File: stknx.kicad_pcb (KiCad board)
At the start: 2 copper layers, 51.3 x 20.3 mm, 51 parts, among them J1 KNX, J2 PMOD, J3 VDDHV, J4 VCCCORE, J5 VDCDC, U1 STKNX

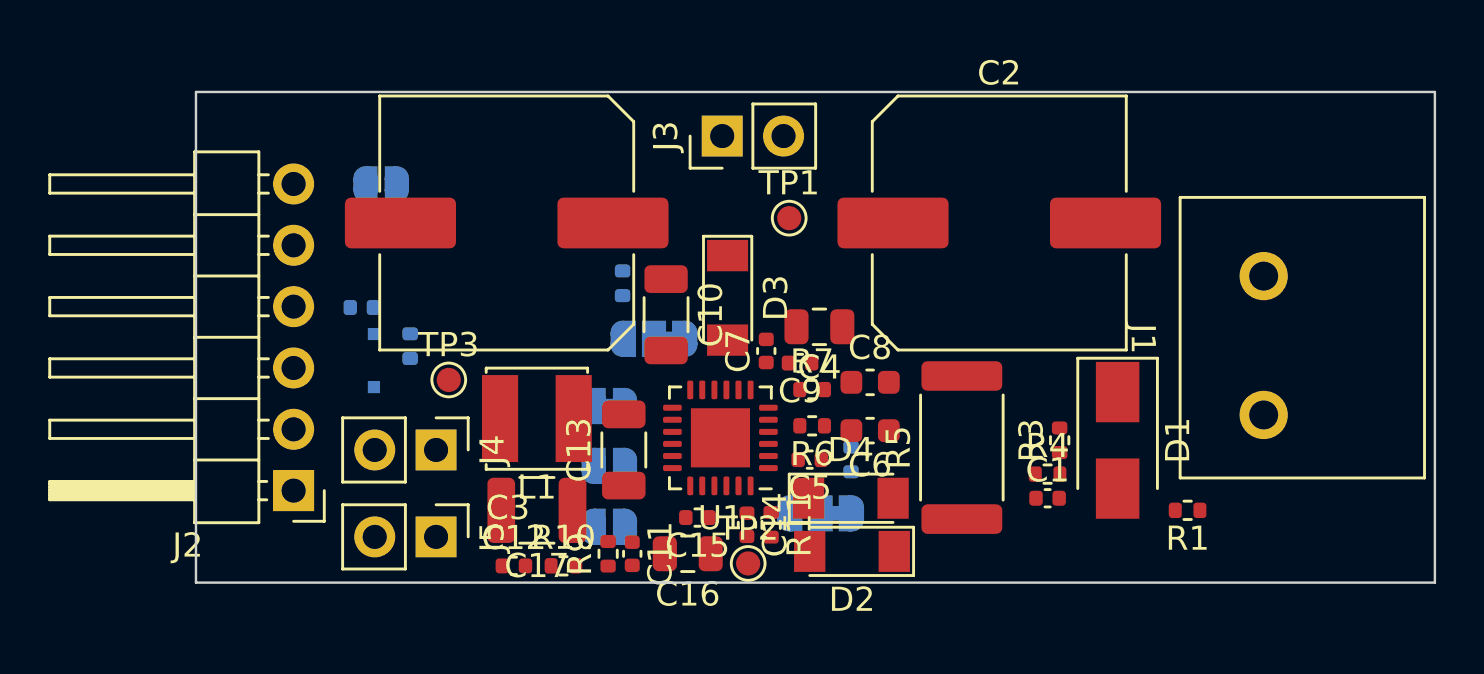
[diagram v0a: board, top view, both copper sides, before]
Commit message: First attempts at routing
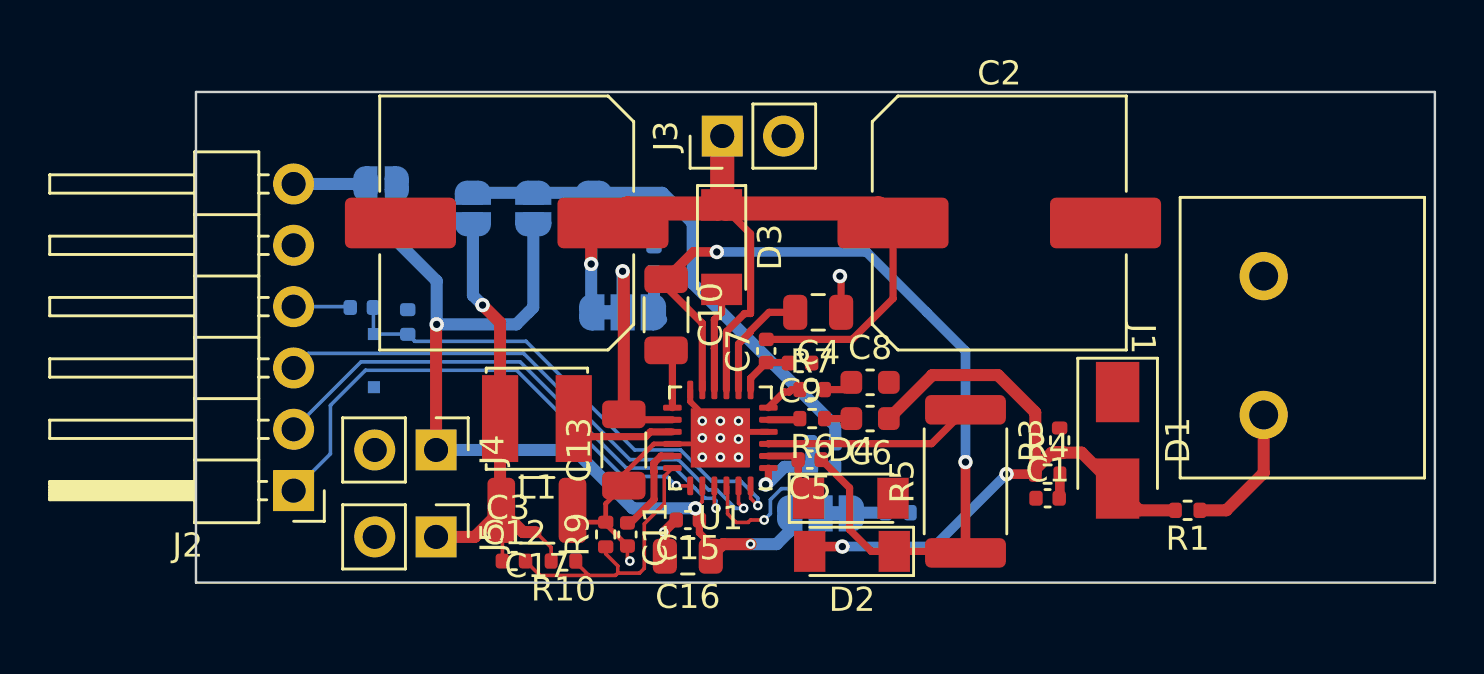
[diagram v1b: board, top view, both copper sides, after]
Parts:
- removed TP1: HV, TestPoint:TestPoint_Pad_D1.0mm
- removed TP2: VCCCORE, TestPoint:TestPoint_Pad_D1.0mm
- removed TP3: VCCDCDC, TestPoint:TestPoint_Pad_D1.0mm
- C14, R11: moved to B.Cu
- moved JP3 14.3 mm to (165.9, 101.6), turned to -90 degrees
- moved JP4 11.1 mm to (168.4, 101.6), turned to -90 degrees
- moved JP2 8.21 mm to (170.9, 101.6), turned to -90 degrees
- moved R11 4.02 mm to (180.4, 111.3), turned to 0 degrees
- moved C14 3.96 mm to (180.4, 112.3), turned to 0 degrees
- moved R8 2.94 mm to (183.5, 114.2), turned to 180 degrees
- moved D3 2.11 mm to (176.2, 103.2)
- moved JP1 1.70 mm to (172.1, 105.9), turned to 0 degrees
- moved R2 1.64 mm to (173.4, 103.7)
- moved R5 1.41 mm to (186.3, 112.9)
- moved R12 1.00 mm to (163.2, 106.3), turned to 90 degrees
- moved C11 0.82 mm to (172.3, 115.1)
- moved R9 0.81 mm to (171.4, 115.1)
- moved C4 0.60 mm to (180.2, 105.9)
- moved C6 0.50 mm to (182.3, 110.3)
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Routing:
- net /VCCCORE: track 0.00 -> 38.9 mm, vias 0 -> 3
- net /VDDHV: track 0.00 -> 38.6 mm, vias 0 -> 1
- net Net-(C10-Pad1): track 0.00 -> 36.7 mm, vias 0 -> 2
- net Net-(C6-Pad1): track 0.00 -> 27.9 mm, vias 0 -> 2
- net /KNX_RX: track 0.00 -> 22.6 mm, vias 0 -> 1
- net /KNX_OK: track 0.00 -> 22.3 mm, vias 0 -> 1
- net /KNX_VCC_OK: track 0.00 -> 21.6 mm, vias 0 -> 1
- net /VDD_REGIN: track 0.00 -> 21.2 mm
- net Net-(C18-Pad1): track 0.00 -> 21.1 mm, vias 0 -> 1
- net /VDCDC: track 0.00 -> 20.9 mm, vias 0 -> 1
- net GND: track 0.00 -> 17.4 mm, vias 0 -> 12
- net Net-(C12-Pad2): track 0.00 -> 12.2 mm
- net /DCDC_IN: track 0.00 -> 9.75 mm, vias 0 -> 1
- net Net-(R5-Pad2): track 0.00 -> 8.75 mm
- net /VCC_SEL: track 0.00 -> 7.05 mm, vias 0 -> 1
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- added copper zone on B.Cu, net GND
- added copper zone on F.Cu, net GND
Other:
- rule pad_to_mask_clearance: 0 -> 0.05

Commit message: Minor fixes
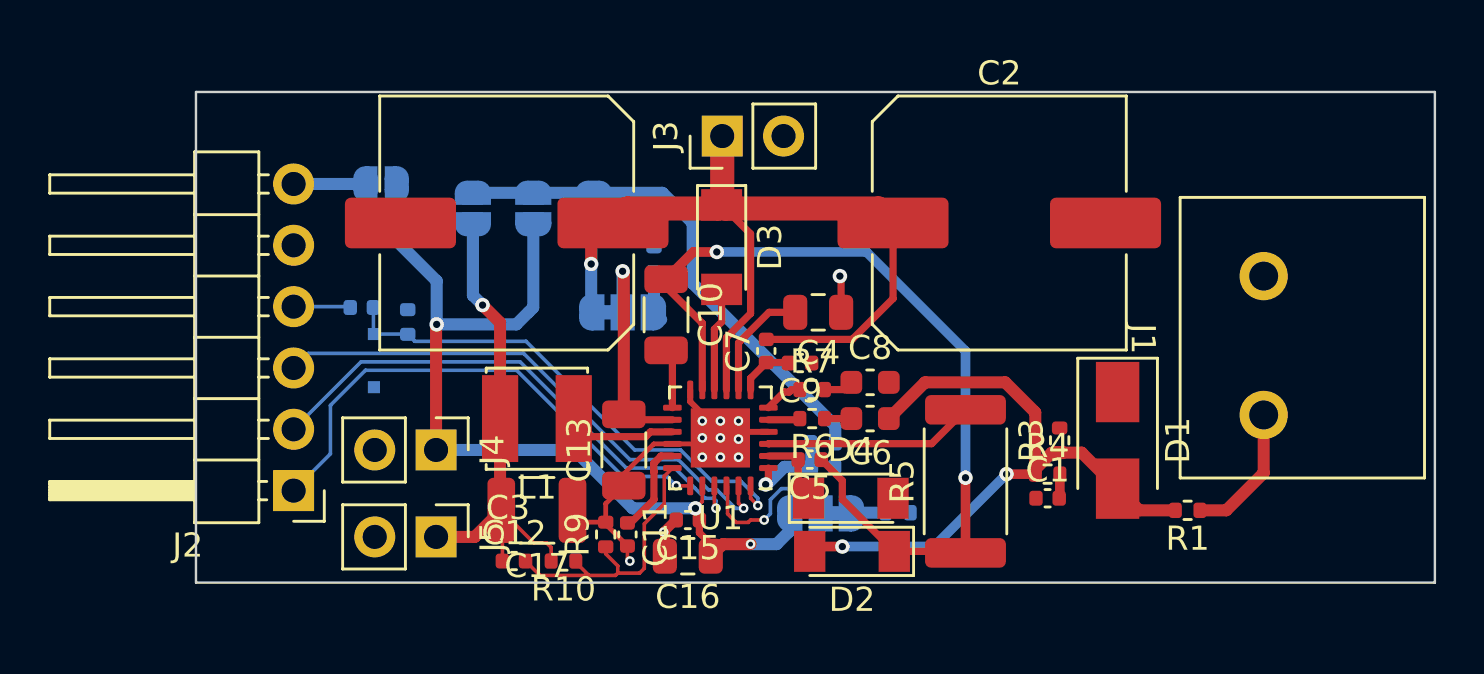
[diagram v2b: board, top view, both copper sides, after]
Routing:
- net Net-(C10-Pad1): track 36.7 -> 36.2 mm
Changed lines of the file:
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@@
   (segment (start 176.35 101.6) (end 176.2 101.45) (width 1) (layer "F.Cu") (net 3))
   (segment (start 183.3 102.2) (end 182.7 101.6) (width 1) (layer "F.Cu") (net 3))
+  (segment (start 176.4 109.1125) (end 176.4 106.95) (width 0.3) (layer "F.Cu") (net 3))
   (segment (start 183.3 105.329776) (end 183.3 102.2) (width 0.3) (layer "F.Cu") (net 3))
-  (segment (start 176.4 109.1125) (end 176.4 106.7) (width 0.3) (layer "F.Cu") (net 3))
+  (segment (start 177.399511 105.950489) (end 177.399511 102.649511) (width 0.3) (layer "F.Cu") (net 3))
   (segment (start 172.3 101.6) (end 176.05 101.6) (width 1) (layer "F.Cu") (net 3))
-  (segment (start 177.399511 105.949511) (end 177.399511 102.649511) (width 0.3) (layer "F.Cu") (net 3))
   (segment (start 170.8 103.9) (end 170.8 103.1) (width 0.5) (layer "F.Cu") (net 3))
+  (segment (start 177.399511 102.649511) (end 176.2 101.45) (width 0.3) (layer "F.Cu") (net 3))
   (segment (start 182.7 101.6) (end 176.35 101.6) (width 1) (layer "F.Cu") (net 3))
-  (segment (start 177.399511 102.649511) (end 176.2 101.45) (width 0.3) (layer "F.Cu") (net 3))
   (segment (start 170.8 103.1) (end 171.7 102.2) (width 0.5) (layer "F.Cu") (net 3))
-  (segment (start 177.150489 105.949511) (end 177.399511 105.949511) (width 0.3) (layer "F.Cu") (net 3))
-  (segment (start 176.4 106.7) (end 177.150489 105.949511) (width 0.3) (layer "F.Cu") (net 3))
   (segment (start 178.05 107.02) (end 181.609776 107.02) (width 0.3) (layer "F.Cu") (net 3))
+  (segment (start 176.4 106.95) (end 177.399511 105.950489) (width 0.3) (layer "F.Cu") (net 3))
   (segment (start 176.05 101.6) (end 176.2 101.45) (width 1) (layer "F.Cu") (net 3))
   (segment (start 176.225 98.6) (end 176.225 101.425) (width 1) (layer "F.Cu") (net 3))
@@
   (segment (start 170.8 105.9) (end 170.8 102.35) (width 0.5) (layer "B.Cu") (net 3))
   (segment (start 170.8 102.35) (end 170.9 102.25) (width 0.5) (layer "B.Cu") (net 3))
-  (segment (start 177.39048 106.673354) (end 178.163834 105.9) (width 0.3) (layer "F.Cu") (net 4))
-  (segment (start 176.9 107.206416) (end 177.39048 106.715936) (width 0.3) (layer "F.Cu") (net 4))
-  (segment (start 176.9 109.1125) (end 176.9 107.206416) (width 0.3) (layer "F.Cu") (net 4))
+  (segment (start 179.05 106.1) (end 179.25 105.9) (width 0.3) (layer "F.Cu") (net 4))
   (segment (start 178.163834 105.9) (end 179.25 105.9) (width 0.3) (layer "F.Cu") (net 4))
-  (segment (start 177.39048 106.715936) (end 177.39048 106.673354) (width 0.3) (layer "F.Cu") (net 4))
-  (segment (start 179.05 106.1) (end 179.25 105.9) (width 0.3) (layer "F.Cu") (net 4))
+  (segment (start 176.9 109.1125) (end 176.9 107.163834) (width 0.3) (layer "F.Cu") (net 4))
+  (segment (start 176.9 107.163834) (end 178.163834 105.9) (width 0.3) (layer "F.Cu") (net 4))
   (segment (start 186.2375 115.8) (end 186.3 115.8625) (width 0.3) (layer "F.Cu") (net 5))
   (segment (start 175.025 103.4) (end 173.9 104.525) (width 0.4) (layer "F.Cu") (net 5))
-  (segment (start 181.5 114.9) (end 182.4 115.8) (width 0.3) (layer "F.Cu") (net 5))
   (segment (start 183.35 115.8) (end 186.2375 115.8) (width 0.3) (layer "F.Cu") (net 5))
   (segment (start 173.9 104.849022) (end 173.9 104.525) (width 0.3) (layer "F.Cu") (net 5))
-  (segment (start 182.4 115.8) (end 183.35 115.8) (width 0.3) (layer "F.Cu") (net 5))
-  (segment (start 186.3 115.8625) (end 186.3 112.1) (width 0.4) (layer "F.Cu") (net 5))
-  (segment (start 180.33 112) (end 181.5 113.17) (width 0.3) (layer "F.Cu") (net 5))
+  (segment (start 181.2 112.87) (end 181.2 113.65) (width 0.3) (layer "F.Cu") (net 5))
   (segment (start 175.4 109.1125) (end 175.4 106.349022) (width 0.3) (layer "F.Cu") (net 5))
+  (segment (start 186.3 115.8625) (end 186.3 112.75) (width 0.4) (layer "F.Cu") (net 5))
   (segment (start 175.4 106.349022) (end 173.9 104.849022) (width 0.3) (layer "F.Cu") (net 5))
   (segment (start 176 103.4) (end 175.025 103.4) (width 0.4) (layer "F.Cu") (net 5))
-  (segment (start 181.5 113.17) (end 181.5 114.9) (width 0.3) (layer "F.Cu") (net 5))
-  (via (at 186.3 112.1) (size 0.6) (drill 0.3) (layers "F.Cu" "B.Cu") (net 5))
+  (segment (start 181.2 113.65) (end 183.35 115.8) (width 0.3) (layer "F.Cu") (net 5))
+  (segment (start 180.33 112) (end 181.2 112.87) (width 0.3) (layer "F.Cu") (net 5))
+  (via (at 186.3 112.75) (size 0.6) (drill 0.3) (layers "F.Cu" "B.Cu") (net 5))
   (via (at 176 103.4) (size 0.6) (drill 0.3) (layers "F.Cu" "B.Cu") (net 5))
-  (segment (start 182.2 103.4) (end 176 103.4) (width 0.4) (layer "B.Cu") (net 5))
-  (segment (start 184.7 105.9) (end 182.2 103.4) (width 0.4) (layer "B.Cu") (net 5))
-  (segment (start 186.3 112.1) (end 186.3 107.5) (width 0.4) (layer "B.Cu") (net 5))
-  (segment (start 186.3 107.5) (end 184.7 105.9) (width 0.4) (layer "B.Cu") (net 5))
+  (segment (start 176 103.4) (end 182.2 103.4) (width 0.4) (layer "B.Cu") (net 5))
+  (segment (start 186.3 107.5) (end 186.3 112.75) (width 0.4) (layer "B.Cu") (net 5))
+  (segment (start 182.2 103.4) (end 186.3 107.5) (width 0.4) (layer "B.Cu") (net 5))
   (segment (start 179.37 112) (end 179.37 113.17) (width 0.3) (layer "F.Cu") (net 6))
   (segment (start 179.22 111.85) (end 179.37 112) (width 0.3) (layer "F.Cu") (net 6))
@@
   (segment (start 188 112.6) (end 189.19 112.6) (width 0.4) (layer "F.Cu") (net 7))
   (segment (start 189.880001 111.71) (end 189.19 112.400001) (width 0.5) (layer "F.Cu") (net 7))
-  (segment (start 184.925 108.5) (end 183.125 110.3) (width 0.5) (layer "F.Cu") (net 7))
+  (segment (start 184.625 108.8) (end 183.125 110.3) (width 0.5) (layer "F.Cu") (net 7))
   (segment (start 194.99 114.1) (end 193.5 114.1) (width 0.5) (layer "F.Cu") (net 7))
+  (segment (start 189.19 110.043802) (end 187.946198 108.8) (width 0.5) (layer "F.Cu") (net 7))
+  (segment (start 191.11 111.71) (end 190.2 111.71) (width 0.5) (layer "F.Cu") (net 7))
   (segment (start 189.19 112.6) (end 189.19 110.043802) (width 0.5) (layer "F.Cu") (net 7))
-  (segment (start 189.19 110.043802) (end 187.646198 108.5) (width 0.5) (layer "F.Cu") (net 7))
-  (segment (start 191.11 111.71) (end 190.2 111.71) (width 0.5) (layer "F.Cu") (net 7))
-  (segment (start 187.646198 108.5) (end 184.925 108.5) (width 0.5) (layer "F.Cu") (net 7))
+  (segment (start 187.946198 108.8) (end 184.625 108.8) (width 0.5) (layer "F.Cu") (net 7))
   (segment (start 179.85 115.8) (end 180.05 115.6) (width 0.4) (layer "F.Cu") (net 7))
   (via (at 181.2 115.6) (size 0.6) (drill 0.3) (layers "F.Cu" "B.Cu") (net 7))
@@
   (segment (start 167.025 110.3) (end 167.025 114.05) (width 0.5) (layer "F.Cu") (net 13))
   (segment (start 165.975 115.2) (end 167.075 114.1) (width 0.5) (layer "F.Cu") (net 13))
+  (segment (start 168.95 115.45) (end 168.425 115.45) (width 0.15) (layer "F.Cu") (net 13))
+  (segment (start 169.14 116.2) (end 169.14 115.64) (width 0.15) (layer "F.Cu") (net 13))
   (segment (start 167.12 114.145) (end 167.075 114.1) (width 0.15) (layer "F.Cu") (net 13))
   (segment (start 167.025 106.325) (end 166.3 105.6) (width 0.5) (layer "F.Cu") (net 13))
-  (segment (start 169.14 115.64) (end 168.5 115) (width 0.15) (layer "F.Cu") (net 13))
-  (segment (start 167.075 114.1) (end 167.975 115) (width 0.5) (layer "F.Cu") (net 13))
+  (segment (start 168.425 115.45) (end 167.075 114.1) (width 0.15) (layer "F.Cu") (net 13))
   (segment (start 167.025 114.05) (end 167.075 114.1) (width 0.5) (layer "F.Cu") (net 13))
   (segment (start 164.375 115.2) (end 165.975 115.2) (width 0.5) (layer "F.Cu") (net 13))
   (segment (start 167.025 110.3) (end 167.025 106.325) (width 0.5) (layer "F.Cu") (net 13))
-  (segment (start 167.975 115) (end 168.5 115) (width 0.5) (layer "F.Cu") (net 13))
+  (segment (start 169.14 115.64) (end 168.95 115.45) (width 0.15) (layer "F.Cu") (net 13))
   (segment (start 167.12 116.2) (end 167.12 114.145) (width 0.15) (layer "F.Cu") (net 13))
-  (segment (start 169.14 116.2) (end 169.14 115.64) (width 0.15) (layer "F.Cu") (net 13))
   (via (at 166.3 105.6) (size 0.6) (drill 0.3) (layers "F.Cu" "B.Cu") (net 13))
   (segment (start 165.9 105.2) (end 166.3 105.6) (width 0.5) (layer "B.Cu") (net 13))
@@
   (segment (start 160.784 105.664) (end 160.82 105.7) (width 0.15) (layer "B.Cu") (net 19))
   (segment (start 158.475 105.664) (end 160.784 105.664) (width 0.15) (layer "B.Cu") (net 19))
-  (segment (start 175.9 109.1125) (end 175.9 107.393584) (width 0.3) (layer "F.Cu") (net 20))
-  (segment (start 175.9 107.393584) (end 175.899511 107.393095) (width 0.3) (layer "F.Cu") (net 20))
-  (segment (start 175.899511 106.200489) (end 176.2 105.9) (width 0.3) (layer "F.Cu") (net 20))
-  (segment (start 176.2 105.9) (end 176.2 104.95) (width 0.3) (layer "F.Cu") (net 20))
-  (segment (start 175.899511 107.393095) (end 175.899511 106.200489) (width 0.3) (layer "F.Cu") (net 20))
+  (segment (start 175.9 109.1125) (end 175.9 106.6) (width 0.3) (layer "F.Cu") (net 20))
+  (segment (start 175.9 106.6) (end 176.2 106.3) (width 0.3) (layer "F.Cu") (net 20))
+  (segment (start 176.2 106.3) (end 176.2 104.95) (width 0.3) (layer "F.Cu") (net 20))
   (segment (start 197.1 114.1) (end 196.01 114.1) (width 0.5) (layer "F.Cu") (net 21))
   (segment (start 198.65 110.15) (end 198.65 112.55) (width 0.5) (layer "F.Cu") (net 21))
